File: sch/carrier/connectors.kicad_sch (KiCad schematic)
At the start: 5 parts, among them J1 USB_C_Receptacle_USB2.0

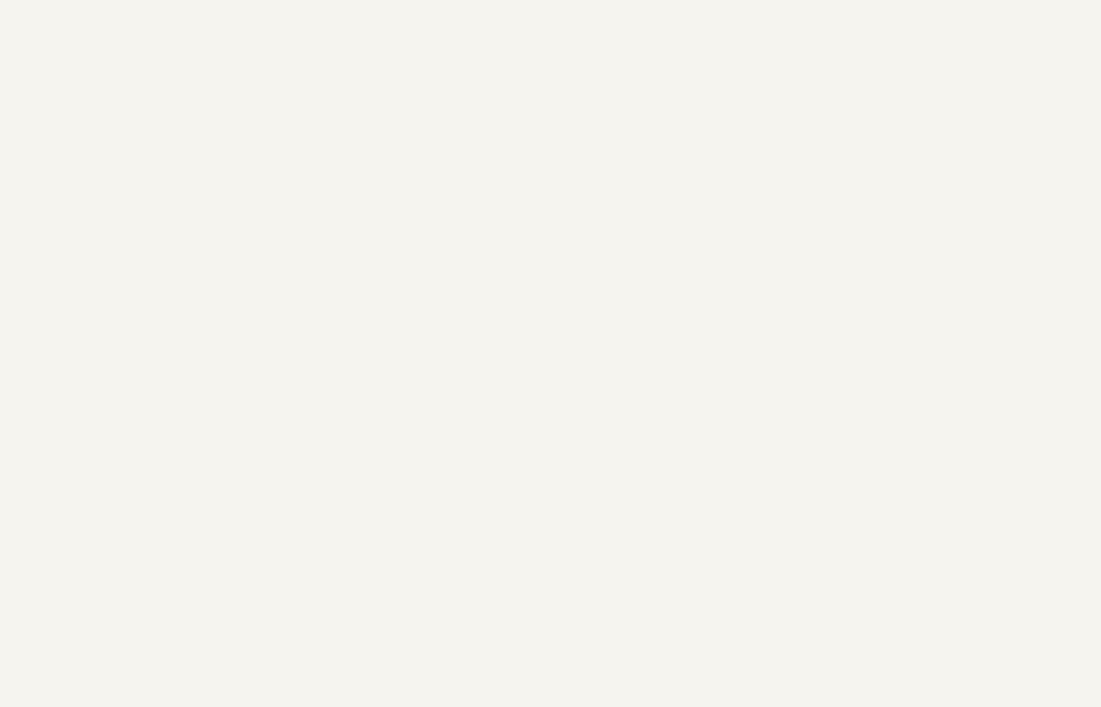
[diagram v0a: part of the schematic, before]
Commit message: get git committed
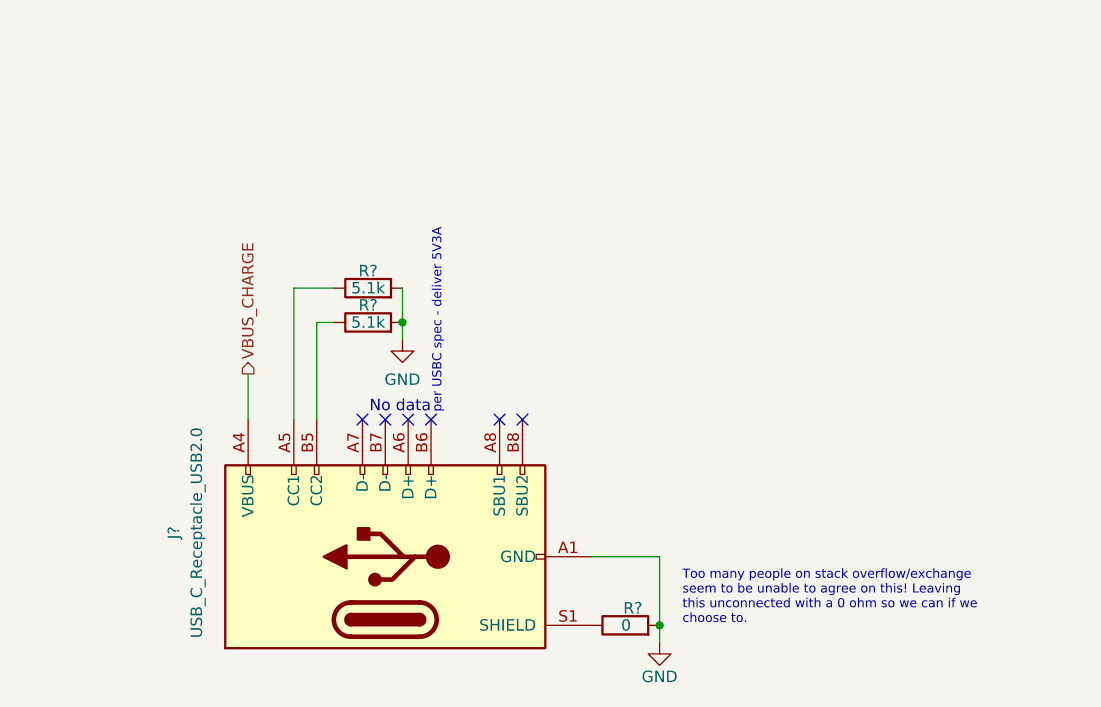
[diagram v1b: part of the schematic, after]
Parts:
- added J?: USB_C_Receptacle_USB2.0, Connector_USB:USB_C_Receptacle_JAE_DX07S016JA1R1500, symbol Connector:USB_C_Receptacle_USB2.0
- added R? (x2): 5.1k, Resistor_SMD:R_0805_2012Metric_Pad1.20x1.40mm_HandSolder, symbol Device:R
- added R?: 0, symbol Device:R
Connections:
- net GND: now also J?.A1 (GND), J?.A12 (GND), J?.B1 (GND), J?.B12 (GND), R?.2, R?.2, R?.2
- new net: J?.A5 (CC1), R?.1
- new net: J?.B5 (CC2), R?.1
- new net: J?.S1 (SHIELD), R?.1
- new net VBUS_CHARGE: J?.A4 (VBUS), J?.A9 (VBUS), J?.B4 (VBUS), J?.B9 (VBUS)
- no-connect marks 2 -> 8
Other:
- note added: "No data"
- note added: "Too many people on stack overflow/exchange seem to be unable to agree on this! Leaving this unconnected with a 0 ohm so we can if we choose to."
- note added: "per USBC spec - deliver 5V3A"
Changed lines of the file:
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@@
   (junction (at 94.615 144.78) (diameter 0.9144) (color 0 0 0 0))
   (junction (at 94.615 147.32) (diameter 0.9144) (color 0 0 0 0))
+  (junction (at 210.82 126.365) (diameter 0.9144) (color 0 0 0 0))
   (junction (at 224.155 66.675) (diameter 0.9144) (color 0 0 0 0))
+  (junction (at 239.395 160.02) (diameter 0.9144) (color 0 0 0 0))
   (junction (at 259.08 28.575) (diameter 0.9144) (color 0 0 0 0))
   (no_connect (at 26.035 27.94))
   (no_connect (at 26.035 30.48))
+  (no_connect (at 206.375 137.16))
+  (no_connect (at 208.915 137.16))
+  (no_connect (at 211.455 137.16))
+  (no_connect (at 213.995 137.16))
+  (no_connect (at 221.615 137.16))
+  (no_connect (at 224.155 137.16))
   (wire (pts (xy 18.415 25.4) (xy 18.415 33.02))
     (stroke (width 0) (type solid) (color 0 0 0 0))
@@
     (stroke (width 0) (type solid) (color 0 0 0 0))
   )
+  (wire (pts (xy 193.675 137.16) (xy 193.675 132.08))
+    (stroke (width 0) (type solid) (color 0 0 0 0))
+  )
+  (wire (pts (xy 198.755 122.555) (xy 198.755 137.16))
+    (stroke (width 0) (type solid) (color 0 0 0 0))
+  )
+  (wire (pts (xy 198.755 122.555) (xy 203.2 122.555))
+    (stroke (width 0) (type solid) (color 0 0 0 0))
+  )
+  (wire (pts (xy 201.295 126.365) (xy 201.295 137.16))
+    (stroke (width 0) (type solid) (color 0 0 0 0))
+  )
+  (wire (pts (xy 203.2 126.365) (xy 201.295 126.365))
+    (stroke (width 0) (type solid) (color 0 0 0 0))
+  )
+  (wire (pts (xy 210.82 122.555) (xy 210.82 126.365))
+    (stroke (width 0) (type solid) (color 0 0 0 0))
+  )
+  (wire (pts (xy 210.82 126.365) (xy 210.82 128.27))
+    (stroke (width 0) (type solid) (color 0 0 0 0))
+  )
   (wire (pts (xy 216.535 66.675) (xy 224.155 66.675))
     (stroke (width 0) (type solid) (color 0 0 0 0))
@@
     (stroke (width 0) (type solid) (color 0 0 0 0))
   )
+  (wire (pts (xy 231.775 152.4) (xy 239.395 152.4))
+    (stroke (width 0) (type solid) (color 0 0 0 0))
+  )
   (wire (pts (xy 239.395 20.955) (xy 244.475 20.955))
     (stroke (width 0) (type solid) (color 0 0 0 0))
@@
   )
   (wire (pts (xy 239.395 28.575) (xy 244.475 28.575))
+    (stroke (width 0) (type solid) (color 0 0 0 0))
+  )
+  (wire (pts (xy 239.395 160.02) (xy 239.395 152.4))
+    (stroke (width 0) (type solid) (color 0 0 0 0))
+  )
+  (wire (pts (xy 239.395 160.02) (xy 239.395 161.925))
     (stroke (width 0) (type solid) (color 0 0 0 0))
   )
@@
     (effects (font (size 1.27 1.27)) (justify left bottom))
   )
+  (text "No data\n" (at 213.995 136.525 180)
+    (effects (font (size 1.27 1.27)) (justify right bottom))
+  )
+  (text "per USBC spec - deliver 5V3A" (at 215.265 136.525 90)
+    (effects (font (size 1.016 1.016)) (justify left bottom))
+  )
+  (text "Too many people on stack overflow/exchange\nseem to be unable to agree on this! Leaving\nthis unconnected with a 0 ohm so we can if we \nchoose to."
+    (at 241.935 160.02 0)
+    (effects (font (size 1.016 1.016)) (justify left bottom))
+  )
   (label "USB2_D-" (at 107.95 27.94 180)
     (effects (font (size 1.27 1.27)) (justify right bottom))
@@
   (label "VBUS" (at 244.475 20.955 180)
     (effects (font (size 1.27 1.27)) (justify right bottom))
+  )
+  (hierarchical_label "VBUS_CHARGE" (shape output) (at 193.675 132.08 90)
+    (effects (font (size 1.27 1.27)) (justify left))
   )
   (symbol (lib_id "power:GND") (at 18.415 161.29 0) (unit 1)
@@
     (pin "1")
   )
+  (symbol (lib_id "power:GND") (at 210.82 128.27 0) (unit 1)
+    (in_bom yes) (on_board yes) (fields_autoplaced)
+    (property "Reference" "#PWR?" (id 0) (at 210.82 134.62 0)
+      (effects (font (size 1.27 1.27)) hide)
+    )
+    (property "Value" "GND" (id 1) (at 210.82 132.715 0))
+    (property "Footprint" "" (id 2) (at 210.82 128.27 0)
+      (effects (font (size 1.27 1.27)) hide)
+    )
+    (property "Datasheet" "" (id 3) (at 210.82 128.27 0)
+      (effects (font (size 1.27 1.27)) hide)
+    )
+    (pin "1")
+  )
   (symbol (lib_id "power:GND") (at 224.155 66.675 0) (unit 1)
     (in_bom yes) (on_board yes) (fields_autoplaced)
@@
     (pin "1")
   )
+  (symbol (lib_id "power:GND") (at 239.395 161.925 0) (unit 1)
+    (in_bom yes) (on_board yes)
+    (property "Reference" "#PWR?" (id 0) (at 239.395 168.275 0)
+      (effects (font (size 1.27 1.27)) hide)
+    )
+    (property "Value" "GND" (id 1) (at 239.395 165.735 0))
+    (property "Footprint" "" (id 2) (at 239.395 161.925 0)
+      (effects (font (size 1.27 1.27)) hide)
+    )
+    (property "Datasheet" "" (id 3) (at 239.395 161.925 0)
+      (effects (font (size 1.27 1.27)) hide)
+    )
+    (pin "1")
+  )
   (symbol (lib_id "power:GND") (at 259.08 28.575 0) (unit 1)
     (in_bom yes) (on_board yes) (fields_autoplaced)
@@
     )
     (pin "1")
+  )
+  (symbol (lib_id "Device:R") (at 207.01 122.555 90) (unit 1)
+    (in_bom yes) (on_board yes)
+    (property "Reference" "R?" (id 0) (at 207.01 120.65 90))
+    (property "Value" "5.1k" (id 1) (at 207.01 122.555 90))
+    (property "Footprint" "Resistor_SMD:R_0805_2012Metric_Pad1.20x1.40mm_HandSolder" (id 2) (at 207.01 124.333 90)
+      (effects (font (size 1.27 1.27)) hide)
+    )
+    (property "Datasheet" "~" (id 3) (at 207.01 122.555 0)
+      (effects (font (size 1.27 1.27)) hide)
+    )
+    (pin "1")
+    (pin "2")
+  )
+  (symbol (lib_id "Device:R") (at 207.01 126.365 90) (unit 1)
+    (in_bom yes) (on_board yes)
+    (property "Reference" "R?" (id 0) (at 207.01 124.46 90))
+    (property "Value" "5.1k" (id 1) (at 207.01 126.365 90))
+    (property "Footprint" "Resistor_SMD:R_0805_2012Metric_Pad1.20x1.40mm_HandSolder" (id 2) (at 207.01 128.143 90)
+      (effects (font (size 1.27 1.27)) hide)
+    )
+    (property "Datasheet" "~" (id 3) (at 207.01 126.365 0)
+      (effects (font (size 1.27 1.27)) hide)
+    )
+    (pin "1")
+    (pin "2")
   )
   (symbol (lib_id "Device:R") (at 216.535 62.865 0) (unit 1)
@@
     )
     (property "Datasheet" "~" (id 3) (at 216.535 62.865 0)
+      (effects (font (size 1.27 1.27)) hide)
+    )
+    (pin "1")
+    (pin "2")
+  )
+  (symbol (lib_id "Device:R") (at 235.585 160.02 90) (unit 1)
+    (in_bom yes) (on_board yes)
+    (property "Reference" "R?" (id 0) (at 237.4899 158.115 90)
+      (effects (font (size 1.27 1.27)) (justify left))
+    )
+    (property "Value" "0" (id 1) (at 236.2199 160.02 90)
+      (effects (font (size 1.27 1.27)) (justify left))
+    )
+    (property "Footprint" "" (id 2) (at 235.585 161.798 90)
+      (effects (font (size 1.27 1.27)) hide)
+    )
+    (property "Datasheet" "~" (id 3) (at 235.585 160.02 0)
       (effects (font (size 1.27 1.27)) hide)
     )
@@
     (pin "2")
   )
+  (symbol (lib_id "Connector:USB_C_Receptacle_USB2.0") (at 208.915 152.4 90) (unit 1)
+    (in_bom yes) (on_board yes) (fields_autoplaced)
+    (property "Reference" "J?" (id 0) (at 185.42 149.733 0))
+    (property "Value" "USB_C_Receptacle_USB2.0" (id 1) (at 187.96 149.733 0))
+    (property "Footprint" "Connector_USB:USB_C_Receptacle_JAE_DX07S016JA1R1500" (id 2) (at 208.915 148.59 0)
+      (effects (font (size 1.27 1.27)) hide)
+    )
+    (property "Datasheet" "https://www.usb.org/sites/default/files/documents/usb_type-c.zip" (id 3) (at 208.915 148.59 0)
+      (effects (font (size 1.27 1.27)) hide)
+    )
+    (pin "A1")
+    (pin "A12")
+    (pin "A4")
+    (pin "A5")
+    (pin "A6")
+    (pin "A7")
+    (pin "A8")
+    (pin "A9")
+    (pin "B1")
+    (pin "B12")
+    (pin "B4")
+    (pin "B5")
+    (pin "B6")
+    (pin "B7")
+    (pin "B8")
+    (pin "B9")
+    (pin "S1")
+  )
   (symbol (lib_id "Connector:USB_C_Receptacle_USB2.0") (at 224.155 36.195 0) (unit 1)

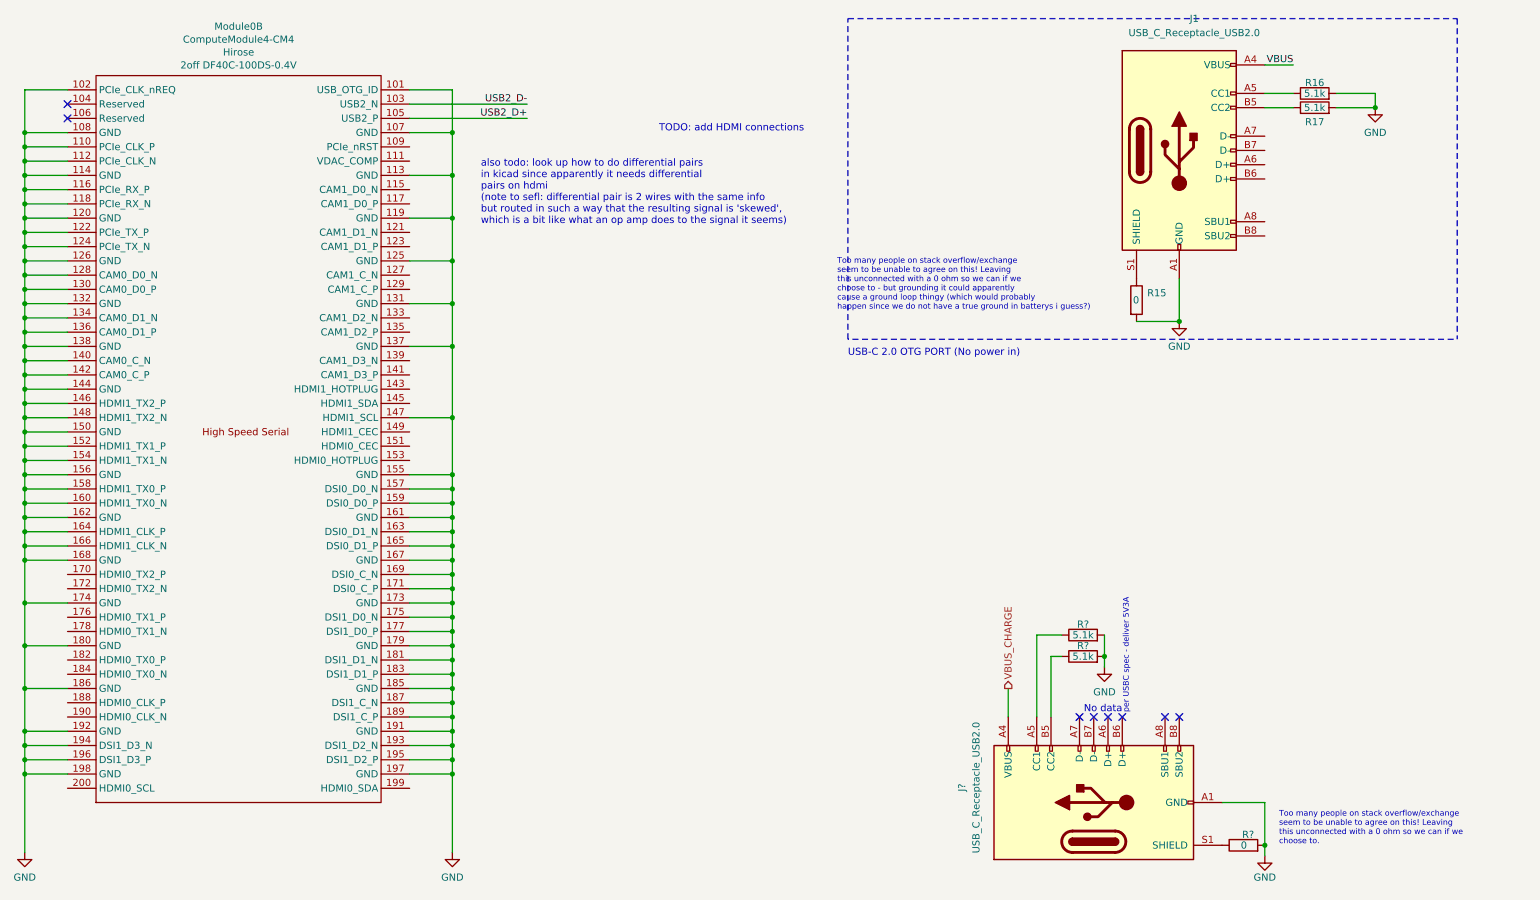
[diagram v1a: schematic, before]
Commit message: aaaaaaaaaaaaaaaa
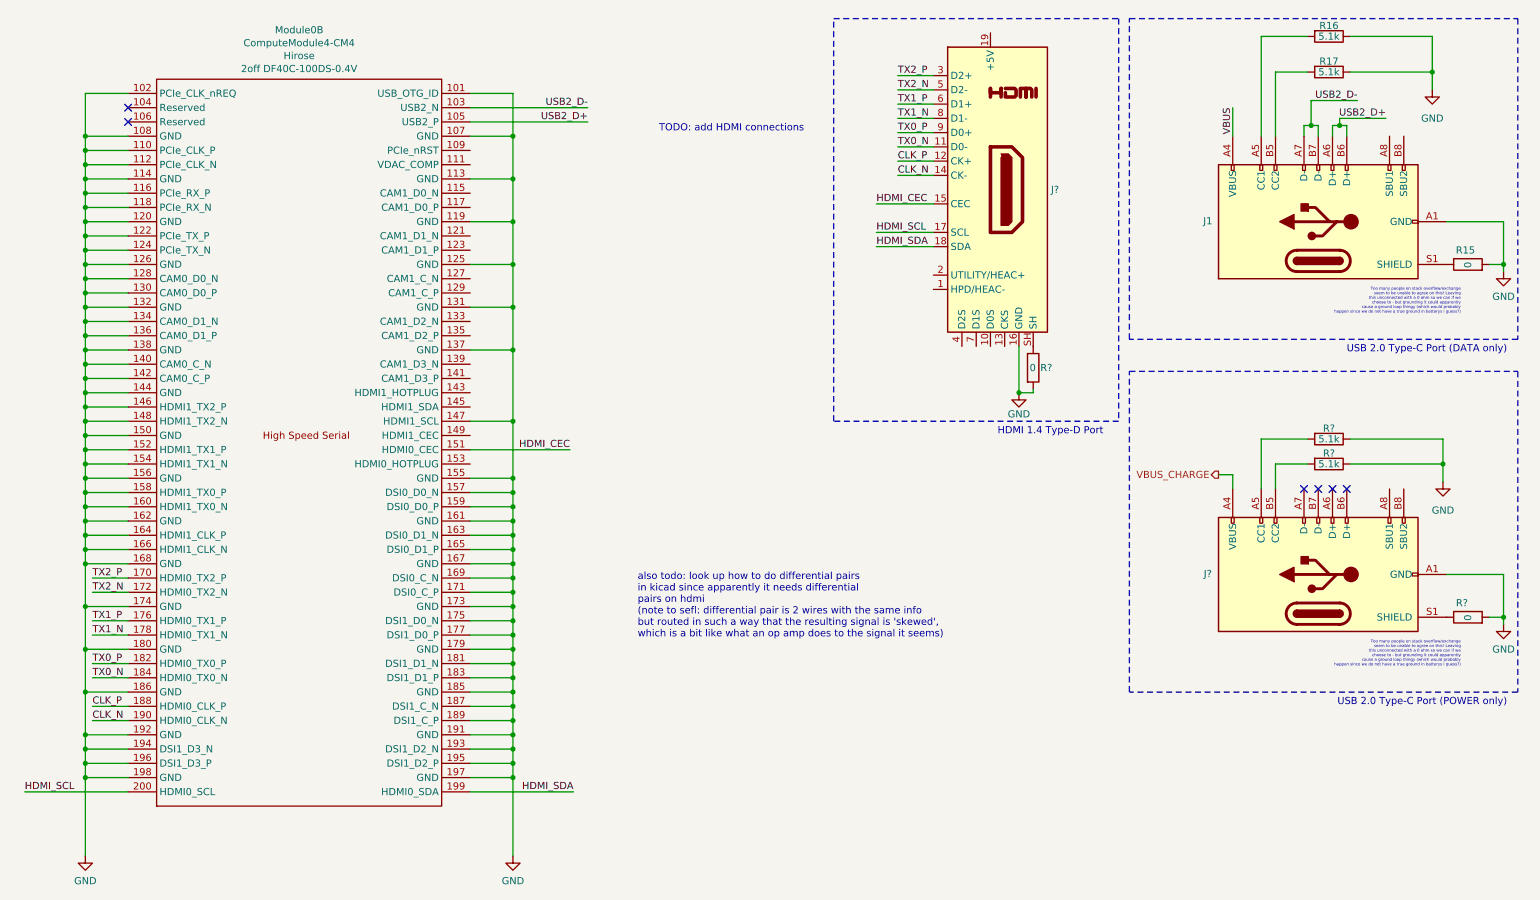
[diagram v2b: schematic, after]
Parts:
- removed J?: USB_C_Receptacle_USB2.0, Connector_USB:USB_C_Receptacle_JAE_DX07S016JA1R1500, symbol Connector:USB_C_Receptacle_USB2.0
- removed R? (x2): 5.1k, Resistor_SMD:R_0805_2012Metric_Pad1.20x1.40mm_HandSolder, symbol Device:R
- removed R?: 0, symbol Device:R
- added J?: HDMI_D_1.4, symbol Connector:HDMI_D_1.4
- added J?: USB_C_Receptacle_USB2.0, Connector_USB:USB_C_Receptacle_JAE_DX07S016JA1R1500, symbol Connector:USB_C_Receptacle_USB2.0
- added R? (x2): 5.1k, Resistor_SMD:R_0805_2012Metric_Pad1.20x1.40mm_HandSolder, symbol Device:R
- added R? (x2): 0, symbol Device:R
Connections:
- net GND: now also R16.1, R17.1, J?.16 (GND), J?.A1 (GND), J?.A12 (GND), J?.B1 (GND), J?.B12 (GND), R?.1, R?.1, R?.2, R?.2; no longer R16.2, R17.2
- net USB2_D+: now also J1.A6 (D+), J1.B6 (D+)
- net USB2_D-: now also J1.A7 (D-), J1.B7 (D-)
- net VBUS_CHARGE: now also J?.A4 (VBUS), J?.A9 (VBUS), J?.B4 (VBUS), J?.B9 (VBUS)
- net at J1.A5 (CC1): now also R16.2; no longer R16.1
- net HDMI_CEC: now reaches Module0.151 (HDMI0_CEC)
- net HDMI_CEC: now also J?.15 (CEC)
- net TX2_P: now reaches Module0.170 (HDMI0_TX2_P)
- net TX2_P: now also J?.3 (D2+)
- net TX2_N: now reaches Module0.172 (HDMI0_TX2_N)
- net TX2_N: now also J?.5 (D2-)
- net TX1_P: now reaches Module0.176 (HDMI0_TX1_P)
- net TX1_P: now also J?.6 (D1+)
- net TX1_N: now reaches Module0.178 (HDMI0_TX1_N)
- net TX1_N: now also J?.8 (D1-)
- net TX0_P: now reaches Module0.182 (HDMI0_TX0_P)
- net TX0_P: now also J?.9 (D0+)
- net TX0_N: now reaches Module0.184 (HDMI0_TX0_N)
- net TX0_N: now also J?.11 (D0-)
- net CLK_P: now reaches Module0.188 (HDMI0_CLK_P)
- net CLK_P: now also J?.12 (CK+)
- net CLK_N: now reaches Module0.190 (HDMI0_CLK_N)
- net CLK_N: now also J?.14 (CK-)
- net HDMI_SDA: now reaches Module0.199 (HDMI0_SDA)
- net HDMI_SDA: now also J?.18 (SDA)
- net HDMI_SCL: now reaches Module0.200 (HDMI0_SCL)
- net HDMI_SCL: now also J?.17 (SCL)
- net at J1.B5 (CC2): now also R17.2; no longer R17.1
- new net: J?.B5 (CC2), R?.2
- new net: J?.SH, R?.1
- new net: J?.S1 (SHIELD), R?.1
- new net: J?.A5 (CC1), R?.2
- no-connect marks 8 -> 6
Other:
- note added: "HDMI 1.4 Type-D Port"
- note added: "USB 2.0 Type-C Port (DATA only)"
- note added: "USB 2.0 Type-C Port (POWER only)"
- note removed: "No data"
- note removed: "Too many people on stack overflow/exchange seem to be unable to agree on this! Leaving this unconnected with a 0 ohm so we can if we choose to."
- note removed: "USB-C 2.0 OTG PORT (No power in)"
- note removed: "per USBC spec - deliver 5V3A"
- moved on the sheet: J1, Module0B, R15, R16, R17
